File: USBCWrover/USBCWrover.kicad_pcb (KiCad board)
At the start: 2 copper layers, 31.5 x 42 mm, 18 parts, among them J1 USB_C_Receptacle_USB2.0, J2 Conn_02x10_Odd_Even, J3 Conn_02x10_Odd_Even, SW1 SW_Push, U1 UMH3N, U2 CP2104, U3 AMS1117-3.3, U4 ESP32-WROVER

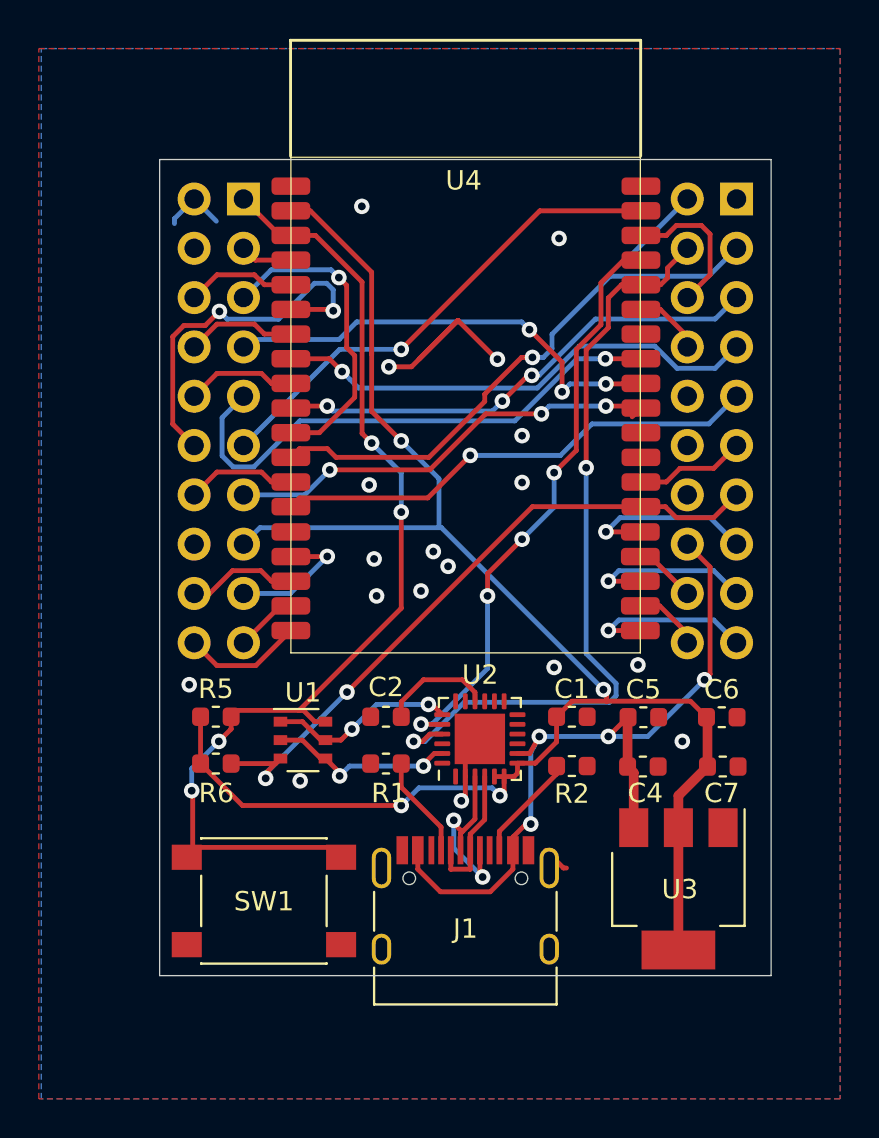
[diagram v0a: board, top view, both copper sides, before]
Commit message: lot prettier
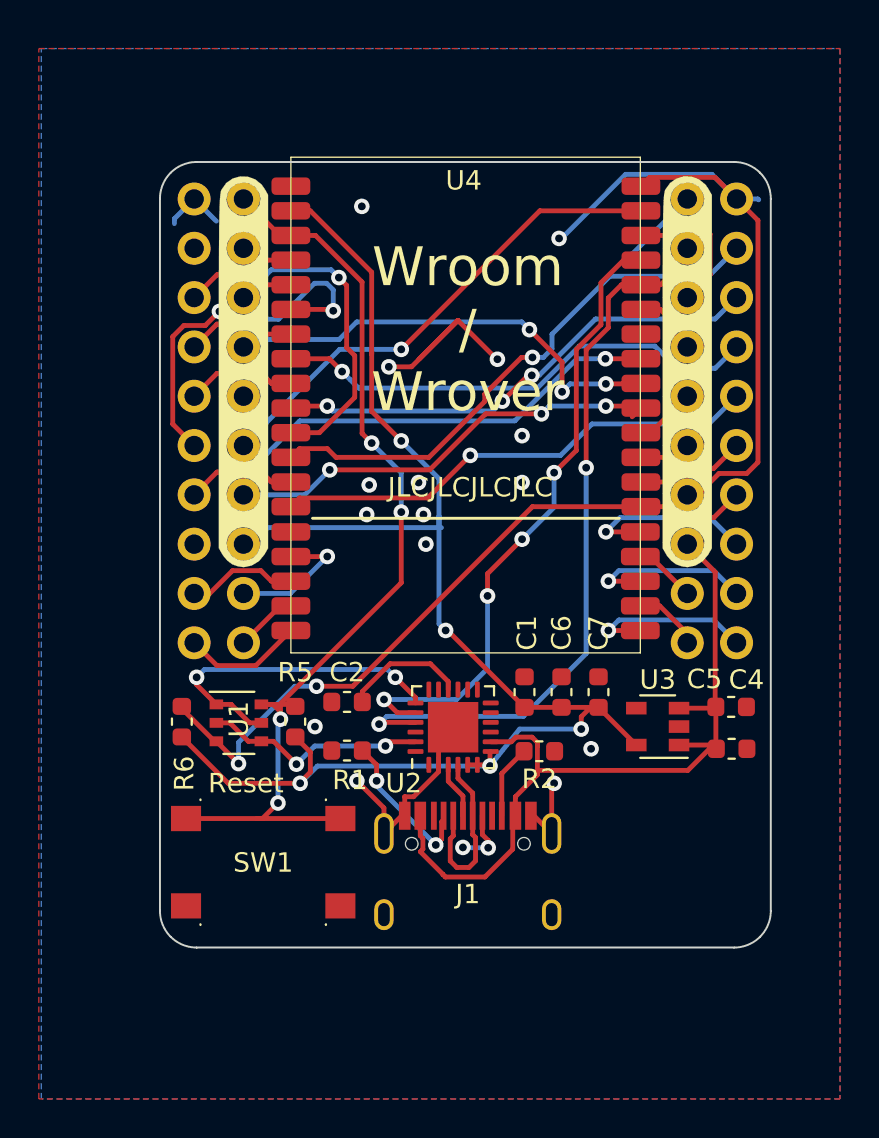
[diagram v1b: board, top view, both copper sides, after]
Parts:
- added G***: LOGO, parts_models:wemos_balkje, B.Cu at (129.5, 115.6)
- added G***: LOGO, parts_models:wemos_balkje, B.Cu at (152.4, 115.6)
- added G***: LOGO, parts_models:wemos_balkje, F.Cu at (129.5, 115.6)
- added G***: LOGO, parts_models:wemos_balkje, F.Cu at (152.4, 115.6)
- U3: value AMS1117-3.3 -> HX9193-33GB; footprint Package_TO_SOT_SMD:SOT-223-3_TabPin2 -> Package_TO_SOT_SMD:SOT-23-5
- moved U3 8.42 mm to (150.9, 133.9), turned to 180 degrees
- moved C6 8.36 mm to (145.9, 132.1), turned to 90 degrees
- moved C7 7.46 mm to (147.8, 132.1), turned to 90 degrees
- moved C4 4.66 mm to (154.7, 135.0)
- moved C5 4.55 mm to (154.7, 132.8)
- moved R5 4.10 mm to (132.2, 133.6), turned to 90 degrees
- moved U1 3.42 mm to (129.3, 133.7)
- moved R6 2.78 mm to (126.4, 133.6), turned to 90 degrees
- moved C1 2.75 mm to (144.0, 132.1), turned to 90 degrees
- moved C2 2.15 mm to (134.9, 132.6)
- moved R1 2.12 mm to (134.9, 135.1)
- moved SW1 2.00 mm to (130.6, 140.8)
- moved R2 1.84 mm to (144.8, 135.1)
- moved J1 1.78 mm to (141.1, 142.5)
- moved U2 1.50 mm to (140.3, 133.9)
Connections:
- J2 pad 10: Net-(J2-Pad10) -> IO17
- J2 pad 12: Net-(J2-Pad12) -> IO16
- U3 pad 1: GND -> +5V
- U3 pad 2: +3V3 -> GND
- U4 pad 27: Net-(U4-Pad27) -> IO16
- U4 pad 28: Net-(U4-Pad28) -> IO17
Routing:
- net GND: track 18.5 -> 64.3 mm, vias 18 -> 15
- net +3V3: track 90.0 -> 78.1 mm, vias 4 -> 5
- net SER_RTS: track 9.71 -> 16.9 mm
- net USB_D+: track 9.85 -> 6.02 mm
- net IO17: track 0.00 -> 3.17 mm
- net ESP_RST: track 53.7 -> 50.8 mm
- net Net-(J1-PadA5): track 5.31 -> 8.10 mm, vias 0 -> 2
- net IO16: track 0.00 -> 2.64 mm
- net USB_D-: track 7.06 -> 9.30 mm
- net ESP_TXD: track 35.0 -> 37.2 mm
- net SER_DTR: track 9.73 -> 11.8 mm
- net ESP_FLS: track 34.9 -> 36.7 mm
- net Net-(J1-PadB5): track 5.56 -> 3.80 mm
- net ESP_RXD: track 40.1 -> 38.3 mm
- net +5V: track 40.6 -> 41.3 mm, vias 4 -> 0
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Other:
- board size 31.5 x 42 mm -> 31.5 x 40.5 mm
- board text added: "JLCJLCJLCJLC"
- board text added: "Reset"
- board text added: "TXD RXD IO22 IO21 IO17* IO16* GND 5V TDD SD0"
- board text added: "Wroom / Wrover"
- board text removed: "TXD RXD IO22 IO21 NC NC GND 5V TDD SD0"
